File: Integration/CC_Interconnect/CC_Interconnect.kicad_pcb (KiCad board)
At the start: 2 copper layers, 66 x 55.9 mm, 7 parts, among them J1 Conn_01x05_Female, J2 Conn_01x05_Female, J3 Conn_01x05_Female, J4 Screw_Terminal_01x02, J5 Conn_01x06_Male, U1 SN74HC32N, U2 SN74LS21N

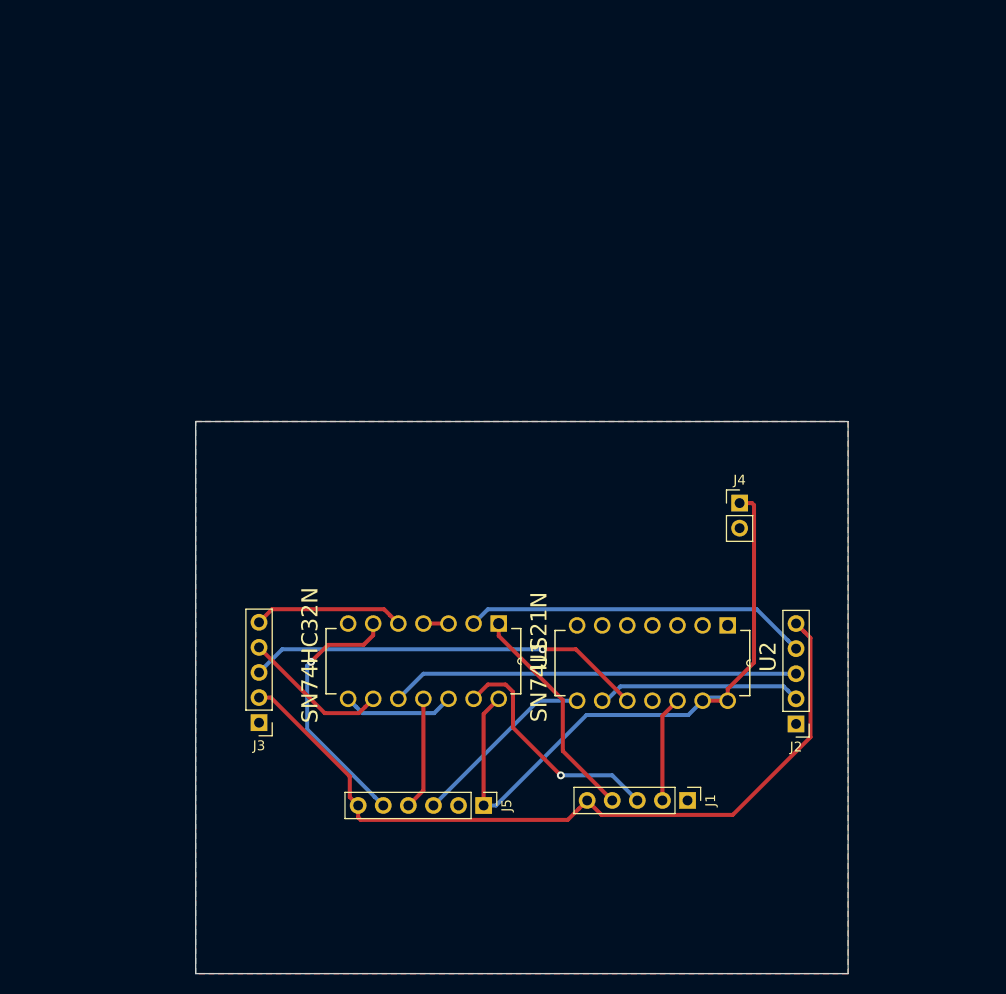
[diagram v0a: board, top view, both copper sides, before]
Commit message: all pcb files are in integration
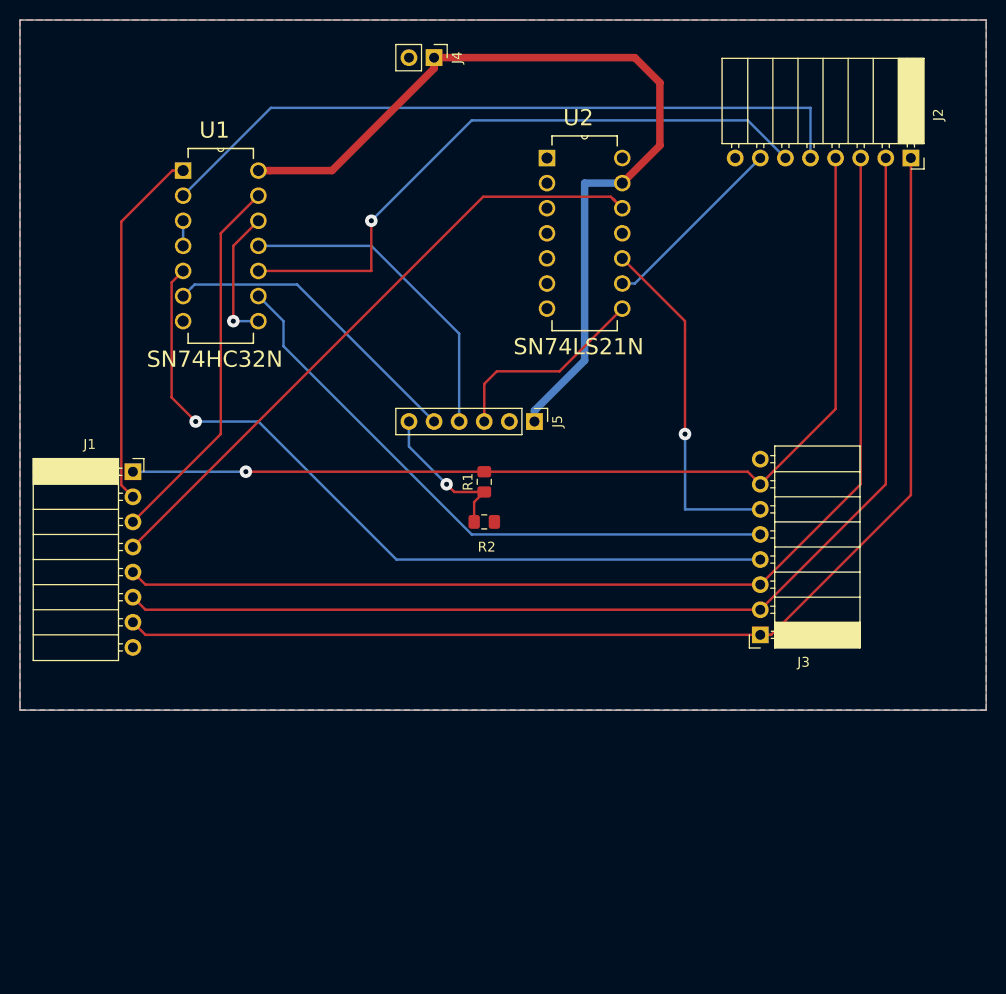
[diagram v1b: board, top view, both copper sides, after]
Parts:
- added R1: 1k, Resistor_SMD:R_0805_2012Metric_Pad1.15x1.40mm_HandSolder, F.Cu at (115.6, 59.4)
- added R2: 2K, Resistor_SMD:R_0805_2012Metric_Pad1.15x1.40mm_HandSolder, F.Cu at (115.6, 63.5)
- J1, J2, J3: value Conn_01x05_Female -> Conn_01x08_Male; footprint Connector_PinHeader_2.54mm:PinHeader_1x05_P2.54mm_Vertical -> Connector_PinSocket_2.54mm:PinSocket_1x08_P2.54mm_Horizontal
- U2: footprint SN74HC32N:DIP254P762X508-14 -> SN74LS21N:DIP254P762X508-14
- moved J1 65.3 mm to (80.0, 58.4), turned to 0 degrees
- moved J2 58.4 mm to (158.8, 26.7), turned to 270 degrees
- moved J4 54.7 mm to (110.5, 16.5), turned to 270 degrees
- moved J3 51.5 mm to (143.5, 74.9)
- moved U2 39.9 mm to (129.5, 41.9), turned to 0 degrees
- moved U1 39.3 mm to (92.7, 43.2), turned to 0 degrees
- moved J5 39.2 mm to (120.7, 53.3)
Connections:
- J1 pad 1: GND -> Net-(J1-Pad1)
- J2 pad 1: GND -> Net-(J1-Pad7)
- J2 pad 2: Net-(J2-Pad2) -> Net-(J1-Pad6)
- J2 pad 3: Net-(J2-Pad3) -> Net-(J1-Pad5)
- J2 pad 4: Net-(J2-Pad4) -> Net-(J1-Pad1)
- J2 pad 5: Net-(J1-Pad5) -> Net-(J2-Pad5)
- J3 pad 1: GND -> Net-(J1-Pad7)
- J3 pad 2: Net-(J1-Pad5) -> Net-(J1-Pad6)
- J3 pad 3: Net-(J3-Pad3) -> Net-(J1-Pad5)
- J4 pad 1: +3V3 -> +5V
- J5 pad 1: +3V3 -> +5V
- J5 pad 6: Net-(J1-Pad5) -> Net-(J5-Pad6)
- U1 pad 1: Net-(J1-Pad4) -> Net-(J1-Pad2)
- U1 pad 10: Net-(J2-Pad3) -> Net-(J2-Pad6)
- U1 pad 14: +3V3 -> +5V
- U1 pad 2: Net-(J2-Pad4) -> Net-(J2-Pad5)
- U1 pad 5: Net-(J3-Pad5) -> Net-(J3-Pad4)
- U1 pad 9: Net-(J3-Pad4) -> Net-(J3-Pad5)
- U2 pad 10: Net-(J3-Pad3) -> Net-(J3-Pad6)
- U2 pad 12: Net-(J1-Pad2) -> Net-(J1-Pad4)
- U2 pad 13: +3V3 -> +5V
- U2 pad 14: +3V3 -> (no net)
- U2 pad 9: Net-(J2-Pad2) -> Net-(J2-Pad7)
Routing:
- net Net-(J1-Pad7): track 0.00 -> 120.3 mm
- net Net-(J1-Pad6): track 0.00 -> 115.0 mm
- net Net-(J1-Pad1): track 0.00 -> 100.2 mm, vias 0 -> 1
- net +5V: track 0.00 -> 88.9 mm
- net Net-(J2-Pad5): track 0.00 -> 72.3 mm
- net +3V3: track 65.5 -> 0.00 mm
- net Net-(J3-Pad4): track 14.9 -> 79.7 mm, vias 0 -> 1
- net Net-(J2-Pad6): track 0.00 -> 64.2 mm, vias 0 -> 1
- net Net-(J3-Pad5): track 15.2 -> 62.3 mm
- net Net-(J1-Pad4): track 22.7 -> 66.1 mm
- net Net-(J2-Pad3): track 41.3 -> 0.00 mm
- net Net-(J3-Pad3): track 40.4 -> 0.00 mm, vias 1 -> 0
- net Net-(J3-Pad6): track 0.00 -> 35.7 mm, vias 0 -> 1
- net Net-(J2-Pad4): track 34.9 -> 0.00 mm
- net Net-(J1-Pad5): track 79.7 -> 111.4 mm
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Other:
- board size 66 x 55.9 mm -> 97.8 x 69.8 mm
- net class Default: clearance 0.4064 -> 0.2; trace_width 0.4064 -> 0.25
- rule trace_clearance: 0.4064 -> 0.2
